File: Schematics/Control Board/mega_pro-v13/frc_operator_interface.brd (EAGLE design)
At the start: 127 x 127 mm, 47 parts, among them CN1 1uF, CN2 1uF, CN3 1uF, CN4 1uF, J1 AVR_SPI_PRG_6PTH, U1 TLC59282_DBQ_24, U4 FT232RLSSOP, Y1 RESONATORSMD

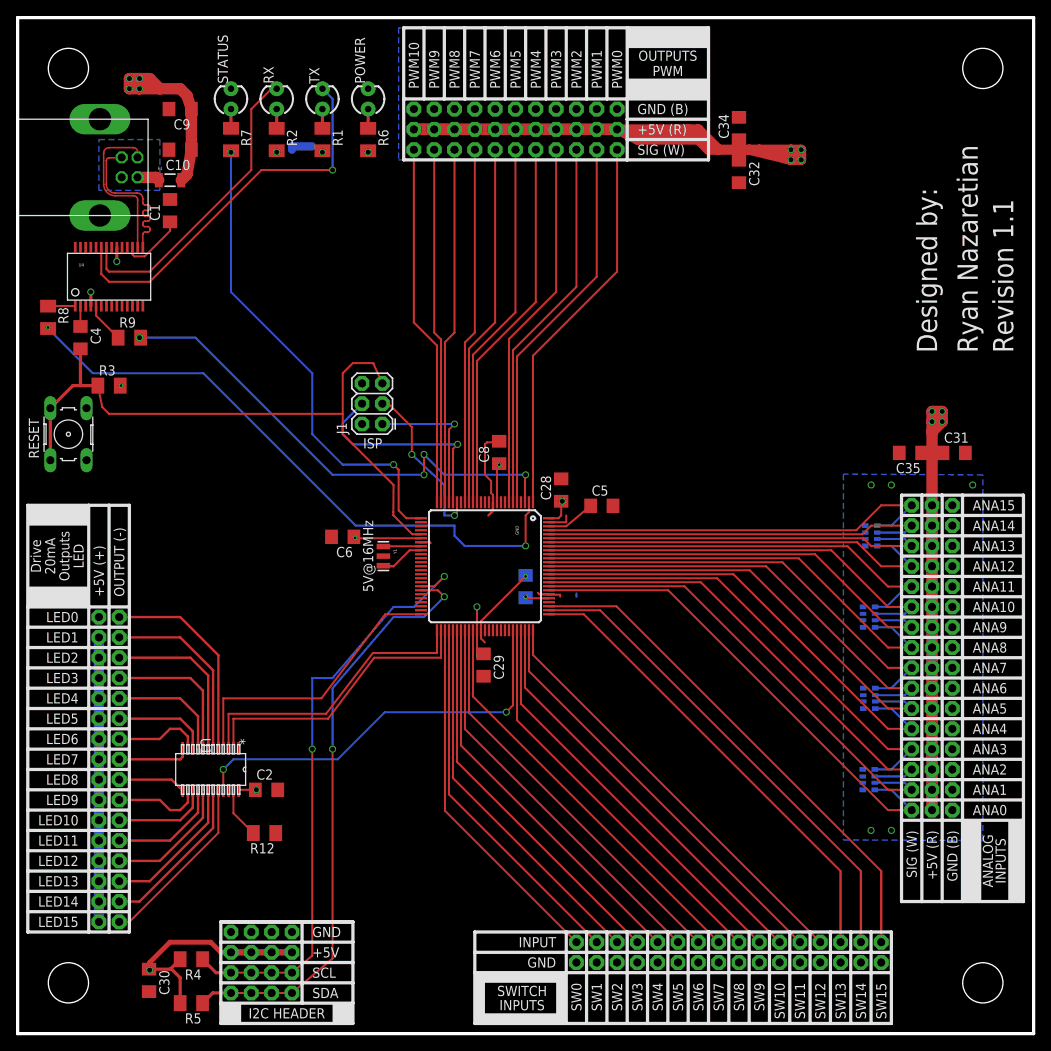
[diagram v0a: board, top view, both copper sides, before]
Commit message: Final control board revision 1.1
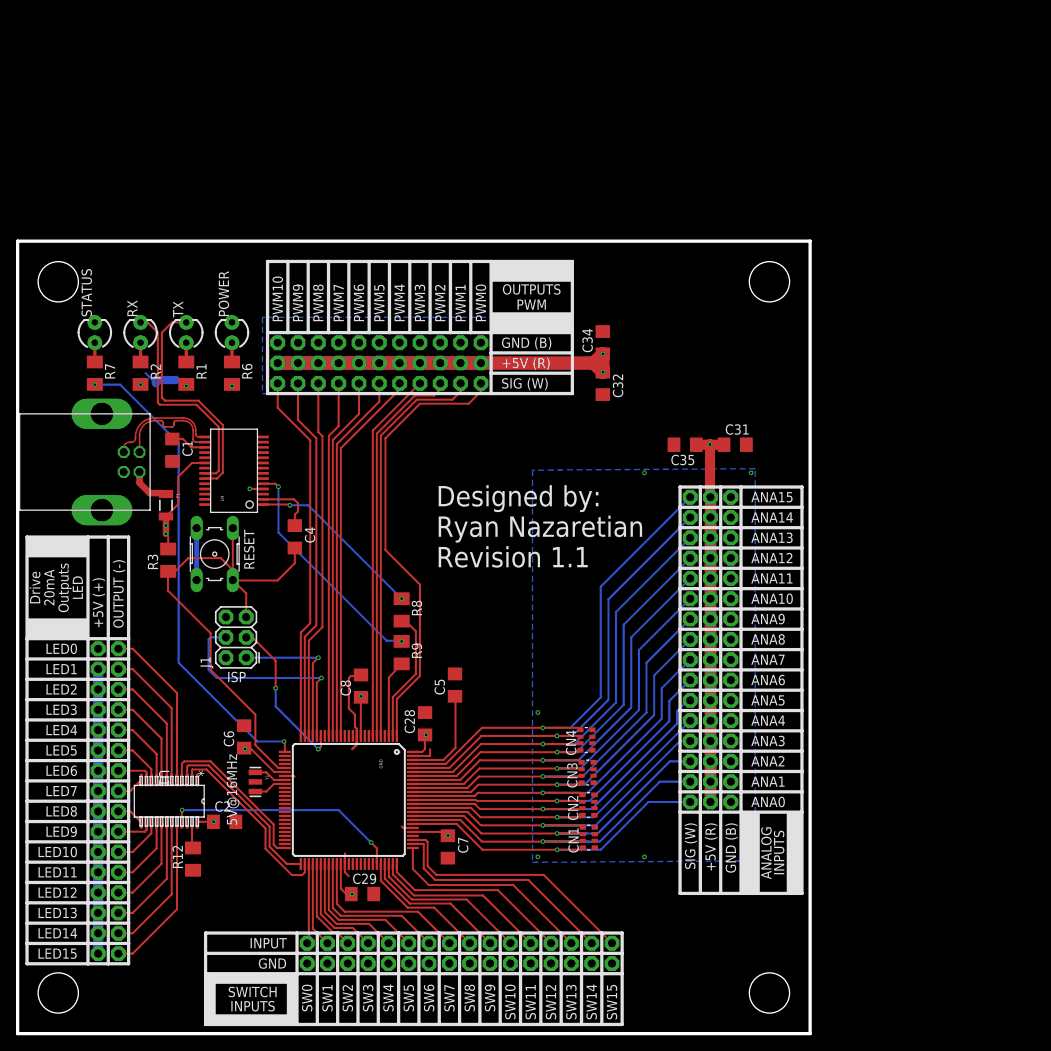
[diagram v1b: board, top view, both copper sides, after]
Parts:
- removed C10, C30: 10uF, rcl:C1206
- removed C9: 0.1uF, rcl:C1206
- removed R4, R5: 10k, rcl:M1206
- removed U$15: I2CHEADER, teamFusion:I2CHEADER
- moved R8 57.4 mm to (48.0, 53.0)
- moved R9 52.0 mm to (48.0, 47.6), turned to 270 degrees
- moved CN4 43.8 mm to (71.1, 36.7), flipped to the top
- moved F1 40.6 mm to (18.5, 66.0), turned to 270 degrees
- moved CN3 40.2 mm to (71.2, 32.6), flipped to the top
- moved CN2 37.6 mm to (71.3, 28.6), flipped to the top
- moved U$14 36.8 mm to (0.25, 77.5)
- moved C4 36.6 mm to (34.7, 62.1)
- moved CN1 35.7 mm to (71.4, 24.5), flipped to the top
- moved C7 34.0 mm to (53.8, 23.3), flipped to the top, turned to 270 degrees
- moved C8 33.9 mm to (42.9, 43.4)
- moved GND 33.8 mm to (41.4, 29.2)
- moved J1 33.8 mm to (28.6, 47.0)
- moved POWER 33.8 mm to (26.8, 87.6)
- moved R1 33.8 mm to (21.1, 82.5)
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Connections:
- net 5V: no longer C10.1, C30.1, C9.1, R4.2, R5.2, U$15.VCC@0, U$15.VCC@1, U$15.VCC@2, U$15.VCC@3
- net DIO20(SDA): no longer R5.1, U$15.SDA@0, U$15.SDA@1, U$15.SDA@2, U$15.SDA@3
- net DIO21(SCL): no longer R4.1, U$15.SCL@0, U$15.SCL@1, U$15.SCL@2, U$15.SCL@3
- net GND: no longer C10.2, C30.2, C9.2, U$15.GND@0, U$15.GND@1, U$15.GND@2, U$15.GND@3
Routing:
- net 5V: track 343.7 -> 245.2 mm, vias 25 -> 15
- net DIO21(SCL): track 75.5 -> 0.00 mm, vias 2 -> 0
- net DIO20(SDA): track 74.5 -> 0.00 mm, vias 2 -> 0
- net DIO0(RX0-I): track 77.8 -> 16.6 mm, vias 2 -> 0
- net DIO1(TX0-O): track 62.5 -> 9.64 mm, vias 4 -> 0
- net DIO36: track 46.6 -> 10.7 mm
- net DIO37: track 45.8 -> 9.99 mm
- net DIO35: track 47.5 -> 11.8 mm
- net DIO34: track 48.3 -> 13.7 mm
- net DIO29: track 50.5 -> 16.4 mm
- net DIO33: track 49.2 -> 15.6 mm
- net DIO28: track 51.3 -> 18.3 mm
- net DIO32: track 50.0 -> 17.5 mm
- net DIO24: track 58.6 -> 26.3 mm
- net DIO23: track 61.4 -> 29.3 mm
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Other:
- board size 127 x 127 mm -> 99.1 x 99.1 mm
